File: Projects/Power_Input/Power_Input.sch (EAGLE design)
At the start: 12 parts, among them U1 SC189ZSKTRT

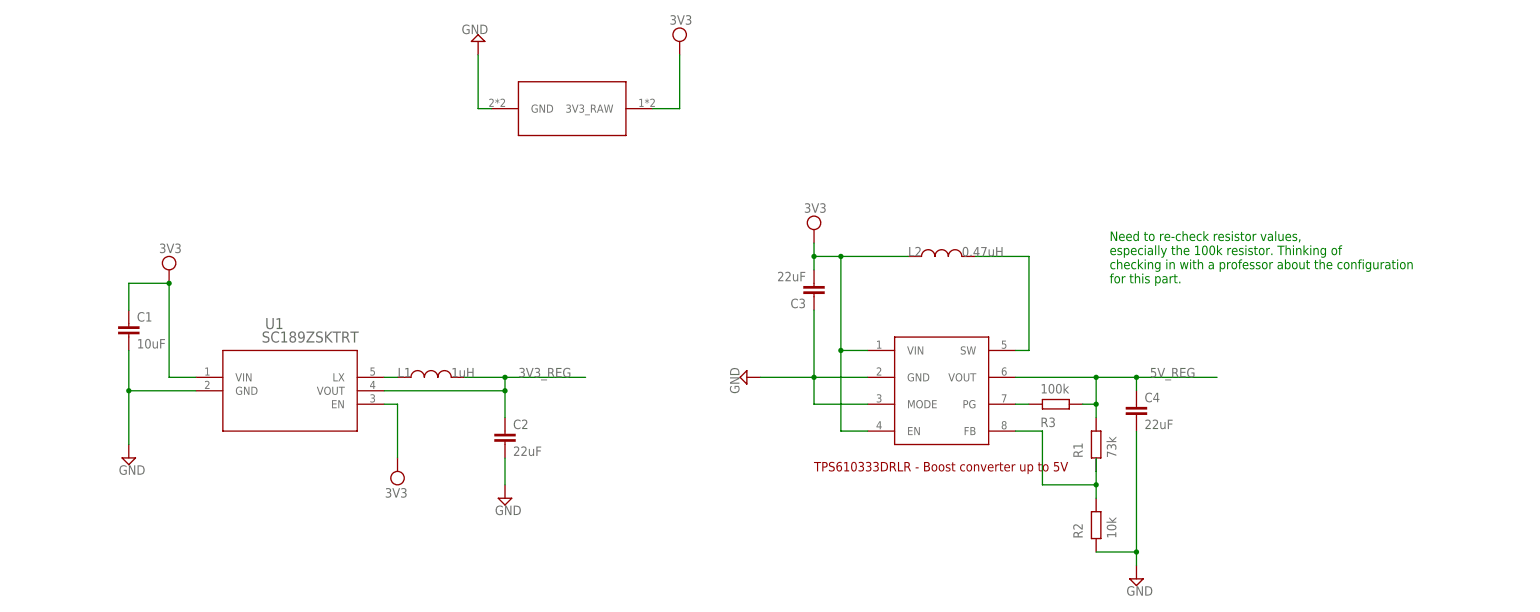
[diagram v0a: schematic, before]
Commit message: Most recent batch of new components
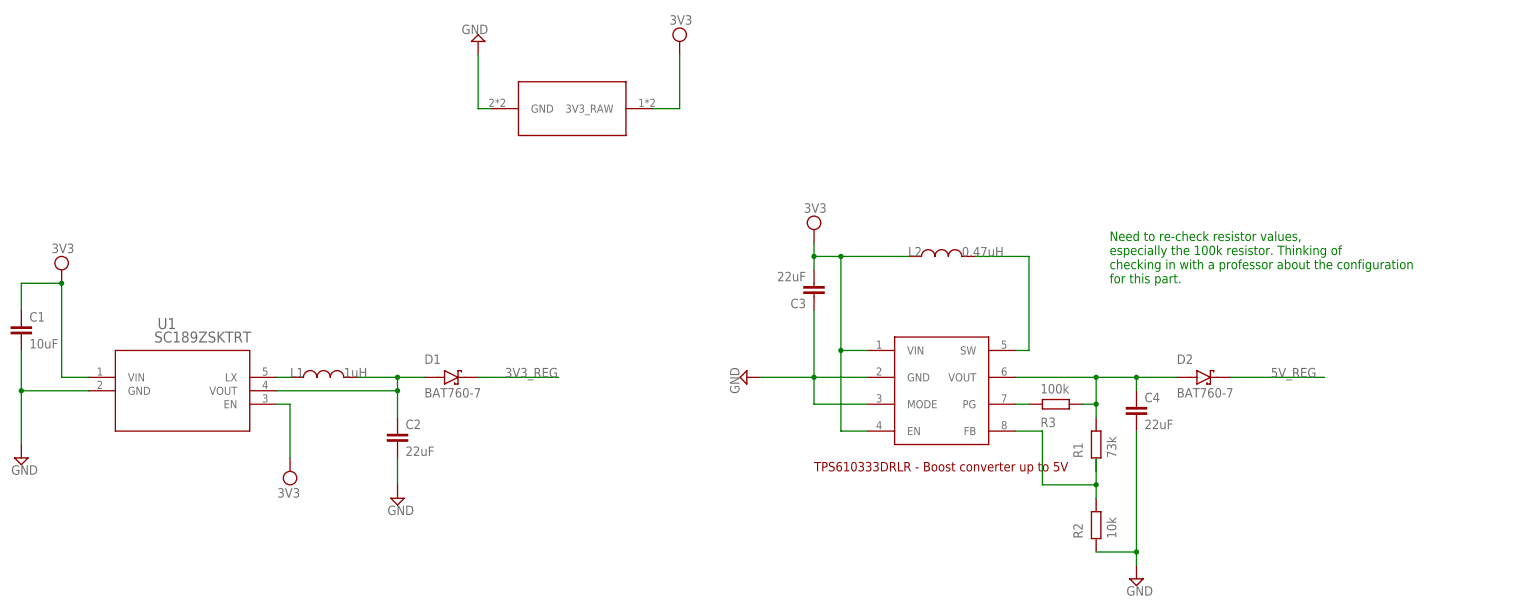
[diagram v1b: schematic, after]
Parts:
- added D1, D2: BAT760-7, BAT760-7:BAT760-7
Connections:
- new net N$4: D1.K
- new net N$6: D2.K
- net 3V3_REG: now also D1.A
- net 5V_REG: now also D2.A
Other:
- moved on the sheet: C1, C2, L1, U1
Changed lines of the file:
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@@
 <part name="R2" library="ngspice-simulation" library_urn="urn:adsk.eagle:library:527439" deviceset="R" device="" value="10k"/>
 <part name="R3" library="ngspice-simulation" library_urn="urn:adsk.eagle:library:527439" deviceset="R" device="" value="100k"/>
+<part name="D1" library="BAT760-7" deviceset="BAT760-7" device=""/>
+<part name="D2" library="BAT760-7" deviceset="BAT760-7" device=""/>
 </parts>
 <sheets>
@@
 <attribute name="VALUE" x="52.705" y="79.375" size="1.778" layer="96" rot="R180"/>
 </instance>
-<instance part="U1" gate="A" x="-5.08" y="12.7" smashed="yes">
-<attribute name="NAME" x="10.5156" y="21.8186" size="2.0828" layer="95" ratio="6" rot="SR0"/>
-<attribute name="VALUE" x="9.8806" y="19.2786" size="2.0828" layer="96" ratio="6" rot="SR0"/>
-</instance>
-<instance part="SUPPLY3" gate="GND" x="-15.24" y="-2.54" smashed="yes">
-<attribute name="VALUE" x="-17.145" y="-5.715" size="1.778" layer="96"/>
-</instance>
-<instance part="SUPPLY4" gate="G$1" x="-7.62" y="33.02" smashed="yes">
-<attribute name="VALUE" x="-9.525" y="36.195" size="1.778" layer="96"/>
-</instance>
-<instance part="C1" gate="G$1" x="-15.24" y="22.86" smashed="yes">
-<attribute name="NAME" x="-13.716" y="23.241" size="1.778" layer="95"/>
-<attribute name="VALUE" x="-13.716" y="18.161" size="1.778" layer="96"/>
-</instance>
-<instance part="SUPPLY5" gate="G$1" x="35.56" y="-5.08" smashed="yes" rot="R180">
-<attribute name="VALUE" x="37.465" y="-8.255" size="1.778" layer="96" rot="R180"/>
-</instance>
-<instance part="L1" gate="G$1" x="40.64" y="12.7" smashed="yes">
-<attribute name="NAME" x="35.56" y="12.7" size="1.778" layer="95"/>
-<attribute name="VALUE" x="45.72" y="12.7" size="1.778" layer="96"/>
-</instance>
-<instance part="C2" gate="G$1" x="55.88" y="2.54" smashed="yes">
-<attribute name="NAME" x="57.404" y="2.921" size="1.778" layer="95"/>
-<attribute name="VALUE" x="57.404" y="-2.159" size="1.778" layer="96"/>
-</instance>
-<instance part="SUPPLY6" gate="GND" x="55.88" y="-10.16" smashed="yes">
-<attribute name="VALUE" x="53.975" y="-13.335" size="1.778" layer="96"/>
+<instance part="U1" gate="A" x="-25.4" y="12.7" smashed="yes">
+<attribute name="NAME" x="-9.8044" y="21.8186" size="2.0828" layer="95" ratio="6" rot="SR0"/>
+<attribute name="VALUE" x="-10.4394" y="19.2786" size="2.0828" layer="96" ratio="6" rot="SR0"/>
+</instance>
+<instance part="SUPPLY3" gate="GND" x="-35.56" y="-2.54" smashed="yes">
+<attribute name="VALUE" x="-37.465" y="-5.715" size="1.778" layer="96"/>
+</instance>
+<instance part="SUPPLY4" gate="G$1" x="-27.94" y="33.02" smashed="yes">
+<attribute name="VALUE" x="-29.845" y="36.195" size="1.778" layer="96"/>
+</instance>
+<instance part="C1" gate="G$1" x="-35.56" y="22.86" smashed="yes">
+<attribute name="NAME" x="-34.036" y="23.241" size="1.778" layer="95"/>
+<attribute name="VALUE" x="-34.036" y="18.161" size="1.778" layer="96"/>
+</instance>
+<instance part="SUPPLY5" gate="G$1" x="15.24" y="-5.08" smashed="yes" rot="R180">
+<attribute name="VALUE" x="17.145" y="-8.255" size="1.778" layer="96" rot="R180"/>
+</instance>
+<instance part="L1" gate="G$1" x="20.32" y="12.7" smashed="yes">
+<attribute name="NAME" x="15.24" y="12.7" size="1.778" layer="95"/>
+<attribute name="VALUE" x="25.4" y="12.7" size="1.778" layer="96"/>
+</instance>
+<instance part="C2" gate="G$1" x="35.56" y="2.54" smashed="yes">
+<attribute name="NAME" x="37.084" y="2.921" size="1.778" layer="95"/>
+<attribute name="VALUE" x="37.084" y="-2.159" size="1.778" layer="96"/>
+</instance>
+<instance part="SUPPLY6" gate="GND" x="35.56" y="-10.16" smashed="yes">
+<attribute name="VALUE" x="33.655" y="-13.335" size="1.778" layer="96"/>
 </instance>
 <instance part="SUPPLY7" gate="G$1" x="114.3" y="40.64" smashed="yes">
@@
 <attribute name="NAME" x="160.02" y="5.08" size="1.778" layer="95" rot="R180"/>
 <attribute name="VALUE" x="162.56" y="11.43" size="1.778" layer="96" rot="R180"/>
+</instance>
+<instance part="D1" gate="G$1" x="45.72" y="12.7" smashed="yes">
+<attribute name="NAME" x="40.64" y="15.24" size="1.778" layer="95"/>
+<attribute name="VALUE" x="40.64" y="8.89" size="1.778" layer="96"/>
+</instance>
+<instance part="D2" gate="G$1" x="187.96" y="12.7" smashed="yes">
+<attribute name="NAME" x="182.88" y="15.24" size="1.778" layer="95"/>
+<attribute name="VALUE" x="182.88" y="8.89" size="1.778" layer="96"/>
 </instance>
 </instances>
@@
 <segment>
 <pinref part="U1" gate="A" pin="GND"/>
-<wire x1="-2.54" y1="10.16" x2="-15.24" y2="10.16" width="0.1524" layer="91"/>
+<wire x1="-22.86" y1="10.16" x2="-35.56" y2="10.16" width="0.1524" layer="91"/>
 <pinref part="SUPPLY3" gate="GND" pin="GND"/>
-<wire x1="-15.24" y1="10.16" x2="-15.24" y2="0" width="0.1524" layer="91"/>
+<wire x1="-35.56" y1="10.16" x2="-35.56" y2="0" width="0.1524" layer="91"/>
 <pinref part="C1" gate="G$1" pin="2"/>
-<wire x1="-15.24" y1="17.78" x2="-15.24" y2="10.16" width="0.1524" layer="91"/>
-<junction x="-15.24" y="10.16"/>
+<wire x1="-35.56" y1="17.78" x2="-35.56" y2="10.16" width="0.1524" layer="91"/>
+<junction x="-35.56" y="10.16"/>
 </segment>
 <segment>
 <pinref part="SUPPLY6" gate="GND" pin="GND"/>
 <pinref part="C2" gate="G$1" pin="2"/>
-<wire x1="55.88" y1="-7.62" x2="55.88" y2="-2.54" width="0.1524" layer="91"/>
+<wire x1="35.56" y1="-7.62" x2="35.56" y2="-2.54" width="0.1524" layer="91"/>
 </segment>
 <segment>
@@
 <pinref part="SUPPLY4" gate="G$1" pin="VDD"/>
 <pinref part="C1" gate="G$1" pin="1"/>
-<wire x1="-7.62" y1="30.48" x2="-15.24" y2="30.48" width="0.1524" layer="91"/>
-<wire x1="-15.24" y1="30.48" x2="-15.24" y2="25.4" width="0.1524" layer="91"/>
+<wire x1="-27.94" y1="30.48" x2="-35.56" y2="30.48" width="0.1524" layer="91"/>
+<wire x1="-35.56" y1="30.48" x2="-35.56" y2="25.4" width="0.1524" layer="91"/>
 <pinref part="U1" gate="A" pin="VIN"/>
-<wire x1="-2.54" y1="12.7" x2="-7.62" y2="12.7" width="0.1524" layer="91"/>
-<wire x1="-7.62" y1="12.7" x2="-7.62" y2="30.48" width="0.1524" layer="91"/>
-<junction x="-7.62" y="30.48"/>
+<wire x1="-22.86" y1="12.7" x2="-27.94" y2="12.7" width="0.1524" layer="91"/>
+<wire x1="-27.94" y1="12.7" x2="-27.94" y2="30.48" width="0.1524" layer="91"/>
+<junction x="-27.94" y="30.48"/>
 </segment>
 <segment>
 <pinref part="U1" gate="A" pin="EN"/>
 <pinref part="SUPPLY5" gate="G$1" pin="VDD"/>
-<wire x1="33.02" y1="7.62" x2="35.56" y2="7.62" width="0.1524" layer="91"/>
-<wire x1="35.56" y1="7.62" x2="35.56" y2="-2.54" width="0.1524" layer="91"/>
+<wire x1="12.7" y1="7.62" x2="15.24" y2="7.62" width="0.1524" layer="91"/>
+<wire x1="15.24" y1="7.62" x2="15.24" y2="-2.54" width="0.1524" layer="91"/>
 </segment>
 <segment>
@@
 <pinref part="U1" gate="A" pin="LX"/>
 <pinref part="L1" gate="G$1" pin="1"/>
-<wire x1="33.02" y1="12.7" x2="35.56" y2="12.7" width="0.1524" layer="91"/>
+<wire x1="12.7" y1="12.7" x2="15.24" y2="12.7" width="0.1524" layer="91"/>
 </segment>
 </net>
@@
 <segment>
 <pinref part="U1" gate="A" pin="VOUT"/>
-<wire x1="33.02" y1="10.16" x2="55.88" y2="10.16" width="0.1524" layer="91"/>
-<wire x1="55.88" y1="10.16" x2="55.88" y2="12.7" width="0.1524" layer="91"/>
-<wire x1="55.88" y1="12.7" x2="71.12" y2="12.7" width="0.1524" layer="91"/>
+<wire x1="12.7" y1="10.16" x2="35.56" y2="10.16" width="0.1524" layer="91"/>
+<wire x1="35.56" y1="10.16" x2="35.56" y2="12.7" width="0.1524" layer="91"/>
 <pinref part="C2" gate="G$1" pin="1"/>
-<wire x1="55.88" y1="5.08" x2="55.88" y2="10.16" width="0.1524" layer="91"/>
-<junction x="55.88" y="10.16"/>
+<wire x1="35.56" y1="5.08" x2="35.56" y2="10.16" width="0.1524" layer="91"/>
+<junction x="35.56" y="10.16"/>
 <pinref part="L1" gate="G$1" pin="2"/>
-<wire x1="48.26" y1="12.7" x2="55.88" y2="12.7" width="0.1524" layer="91"/>
-<junction x="55.88" y="12.7"/>
-<label x="58.42" y="12.7" size="1.778" layer="95"/>
+<wire x1="27.94" y1="12.7" x2="35.56" y2="12.7" width="0.1524" layer="91"/>
+<label x="55.88" y="12.7" size="1.778" layer="95"/>
+<pinref part="D1" gate="G$1" pin="A"/>
+<wire x1="40.64" y1="12.7" x2="35.56" y2="12.7" width="0.1524" layer="91"/>
+<junction x="35.56" y="12.7"/>
 </segment>
 </net>
@@
 <wire x1="167.64" y1="12.7" x2="175.26" y2="12.7" width="0.1524" layer="91"/>
 <wire x1="175.26" y1="12.7" x2="175.26" y2="10.16" width="0.1524" layer="91"/>
-<wire x1="175.26" y1="12.7" x2="190.5" y2="12.7" width="0.1524" layer="91"/>
-<junction x="175.26" y="12.7"/>
 <wire x1="167.64" y1="5.08" x2="167.64" y2="7.62" width="0.1524" layer="91"/>
 <junction x="167.64" y="12.7"/>
@@
 <wire x1="165.1" y1="7.62" x2="167.64" y2="7.62" width="0.1524" layer="91"/>
 <junction x="167.64" y="7.62"/>
-<label x="177.8" y="12.7" size="1.778" layer="95"/>
+<label x="200.66" y="12.7" size="1.778" layer="95"/>
+<pinref part="D2" gate="G$1" pin="A"/>
+<wire x1="182.88" y1="12.7" x2="175.26" y2="12.7" width="0.1524" layer="91"/>
+<junction x="175.26" y="12.7"/>
 </segment>
 </net>
@@
 </segment>
 </net>
+<net name="N$4" class="0">
+<segment>
+<pinref part="D1" gate="G$1" pin="K"/>
+<wire x1="50.8" y1="12.7" x2="66.04" y2="12.7" width="0.1524" layer="91"/>
+</segment>
+</net>
+<net name="N$6" class="0">
+<segment>
+<pinref part="D2" gate="G$1" pin="K"/>
+<wire x1="193.04" y1="12.7" x2="210.82" y2="12.7" width="0.1524" layer="91"/>
+</segment>
+</net>
